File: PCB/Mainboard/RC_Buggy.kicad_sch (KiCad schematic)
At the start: 12 parts, among them SW1 SW_Push, SW2 SW_Push, U1 ESP32-S3-WROOM-1

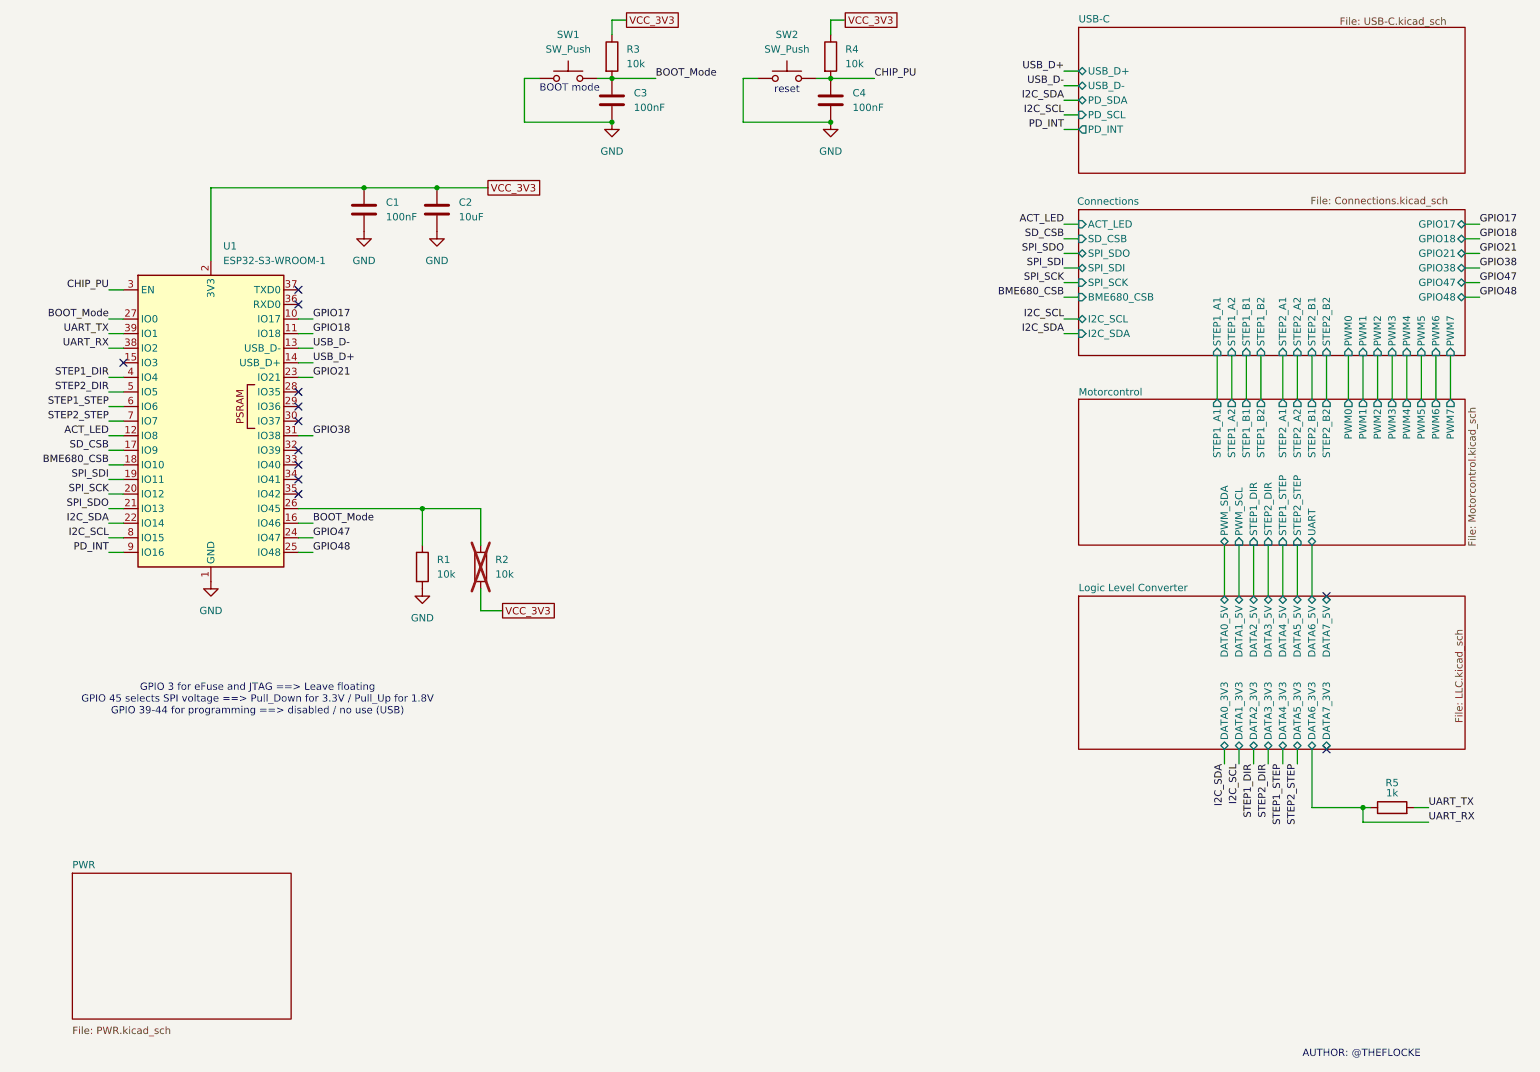
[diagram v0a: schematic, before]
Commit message: Fixed Grammar
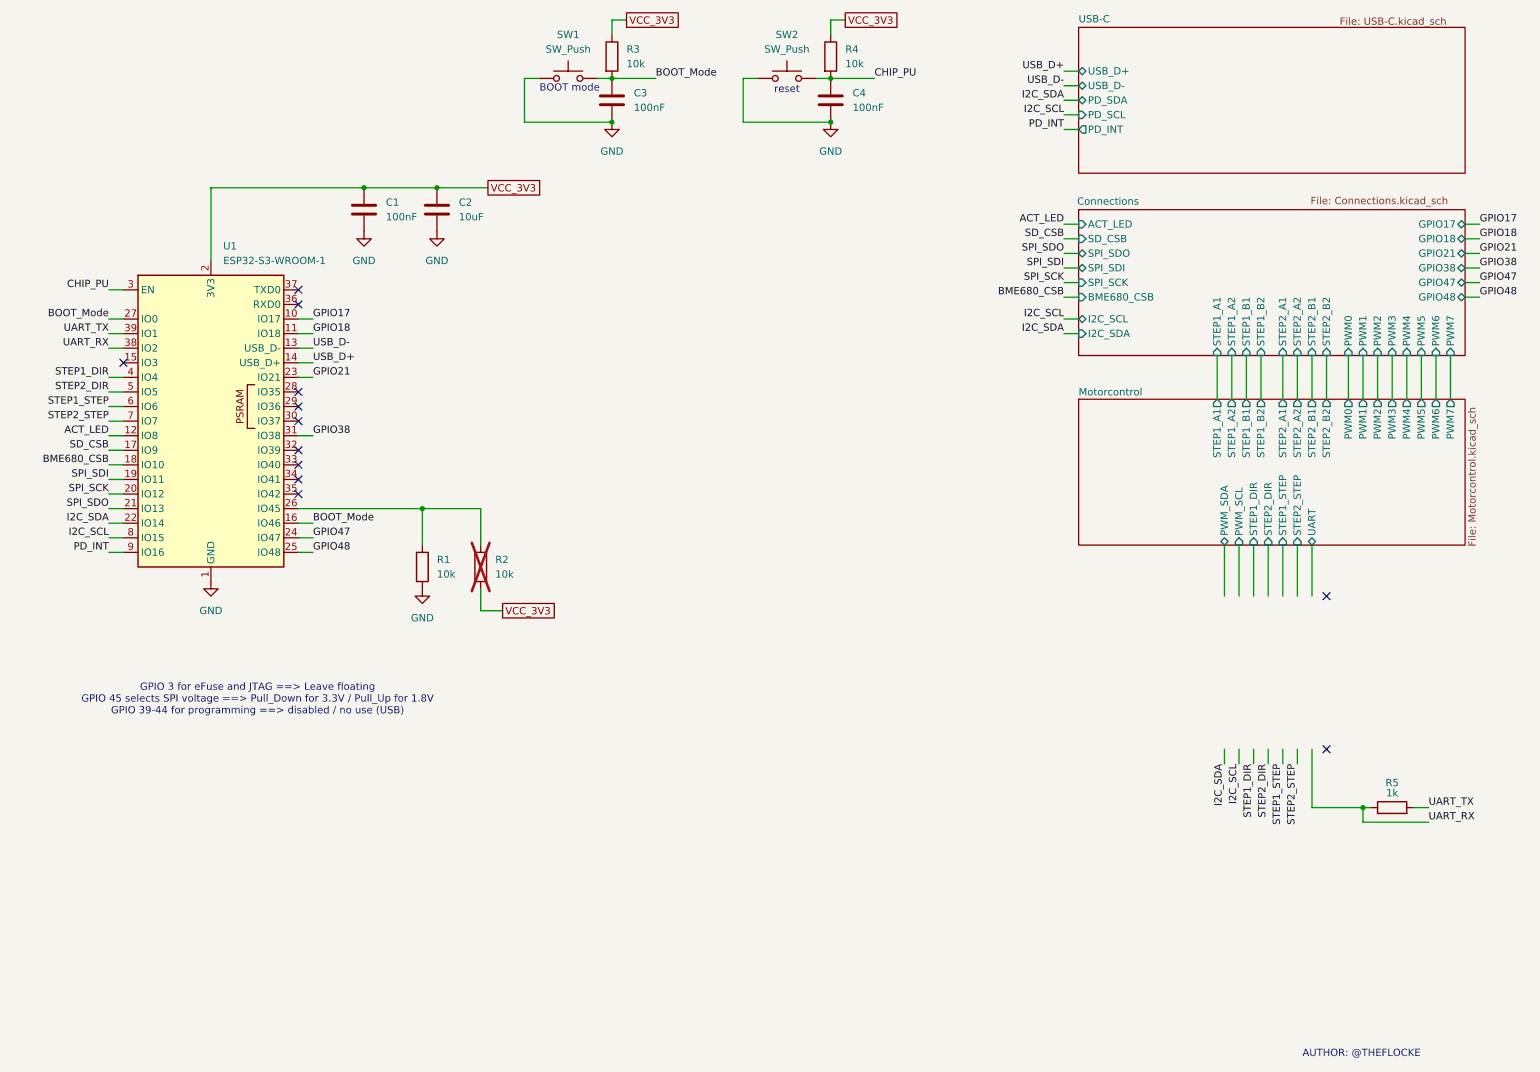
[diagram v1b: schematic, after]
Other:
- removed sheet Logic Level Converter
- removed sheet PWR
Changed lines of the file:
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@@
-	)
-	(sheet
-		(at 25.4 165.1)
-		(size 38.1 25.4)
-		(exclude_from_sim no)
-		(in_bom yes)
-		(on_board yes)
-		(dnp no)
-		(stroke
-			(width 0.1524)
-			(type solid)
-		)
-		(fill
-			(color 0 0 0 0.0000)
-		)
-		(property "Sheetname" "PWR"
-			(at 25.4 164.3884 0)
-			(effects
-				(font
-					(size 1.27 1.27)
-				)
-				(justify left bottom)
-			)
-		)
-		(property "Sheetfile" "PWR.kicad_sch"
-			(at 25.4 191.77 0)
-			(effects
-				(font
-					(size 1.27 1.27)
-				)
-				(justify left top)
-			)
-		)
-		(instances
-			(project "RC_Buggy"
-				(path "/95edd31c-9fee-4eef-843b-c880bdcf4bfe"
-					(page "3")
-				)
-			)
-		)
-	)
-	(sheet
-		(at 200.66 116.84)
-		(size 67.31 26.67)
-		(exclude_from_sim no)
-		(in_bom yes)
-		(on_board yes)
-		(dnp no)
-		(stroke
-			(width 0.1524)
-			(type solid)
-		)
-		(fill
-			(color 0 0 0 0.0000)
-		)
-		(property "Sheetname" "Logic Level Converter"
-			(at 200.66 116.1284 0)
-			(effects
-				(font
-					(size 1.27 1.27)
-				)
-				(justify left bottom)
-			)
-		)
-		(property "Sheetfile" "LLC.kicad_sch"
-			(at 266.192 138.938 90)
-			(effects
-				(font
-					(size 1.27 1.27)
-				)
-				(justify left top)
-			)
-		)
-		(pin "DATA2_5V" bidirectional
-			(at 231.14 116.84 90)
-			(effects
-				(font
-					(size 1.27 1.27)
-				)
-				(justify right)
-			)
-		)
-		(pin "DATA2_3V3" bidirectional
-			(at 231.14 143.51 270)
-			(effects
-				(font
-					(size 1.27 1.27)
-				)
-				(justify left)
-			)
-		)
-		(pin "DATA0_5V" bidirectional
-			(at 226.06 116.84 90)
-			(effects
-				(font
-					(size 1.27 1.27)
-				)
-				(justify right)
-			)
-		)
-		(pin "DATA0_3V3" bidirectional
-			(at 226.06 143.51 270)
-			(effects
-				(font
-					(size 1.27 1.27)
-				)
-				(justify left)
-			)
-		)
-		(pin "DATA7_3V3" bidirectional
-			(at 243.84 143.51 270)
-			(effects
-				(font
-					(size 1.27 1.27)
-				)
-				(justify left)
-			)
-		)
-		(pin "DATA6_3V3" bidirectional
-			(at 241.3 143.51 270)
-			(effects
-				(font
-					(size 1.27 1.27)
-				)
-				(justify left)
-			)
-		)
-		(pin "DATA1_3V3" bidirectional
-			(at 228.6 143.51 270)
-			(effects
-				(font
-					(size 1.27 1.27)
-				)
-				(justify left)
-			)
-		)
-		(pin "DATA3_3V3" bidirectional
-			(at 233.68 143.51 270)
-			(effects
-				(font
-					(size 1.27 1.27)
-				)
-				(justify left)
-			)
-		)
-		(pin "DATA5_3V3" bidirectional
-			(at 238.76 143.51 270)
-			(effects
-				(font
-					(size 1.27 1.27)
-				)
-				(justify left)
-			)
-		)
-		(pin "DATA4_3V3" bidirectional
-			(at 236.22 143.51 270)
-			(effects
-				(font
-					(size 1.27 1.27)
-				)
-				(justify left)
-			)
-		)
-		(pin "DATA4_5V" bidirectional
-			(at 236.22 116.84 90)
-			(effects
-				(font
-					(size 1.27 1.27)
-				)
-				(justify right)
-			)
-		)
-		(pin "DATA7_5V" bidirectional
-			(at 243.84 116.84 90)
-			(effects
-				(font
-					(size 1.27 1.27)
-				)
-				(justify right)
-			)
-		)
-		(pin "DATA6_5V" bidirectional
-			(at 241.3 116.84 90)
-			(effects
-				(font
-					(size 1.27 1.27)
-				)
-				(justify right)
-			)
-		)
-		(pin "DATA1_5V" bidirectional
-			(at 228.6 116.84 90)
-			(effects
-				(font
-					(size 1.27 1.27)
-				)
-				(justify right)
-			)
-		)
-		(pin "DATA3_5V" bidirectional
-			(at 233.68 116.84 90)
-			(effects
-				(font
-					(size 1.27 1.27)
-				)
-				(justify right)
-			)
-		)
-		(pin "DATA5_5V" bidirectional
-			(at 238.76 116.84 90)
-			(effects
-				(font
-					(size 1.27 1.27)
-				)
-				(justify right)
-			)
-		)
-		(instances
-			(project "RC_Buggy"
-				(path "/95edd31c-9fee-4eef-843b-c880bdcf4bfe"
-					(page "4")
-				)
-			)
-		)
 	)
 	(sheet

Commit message: upload images and deleted pcb new
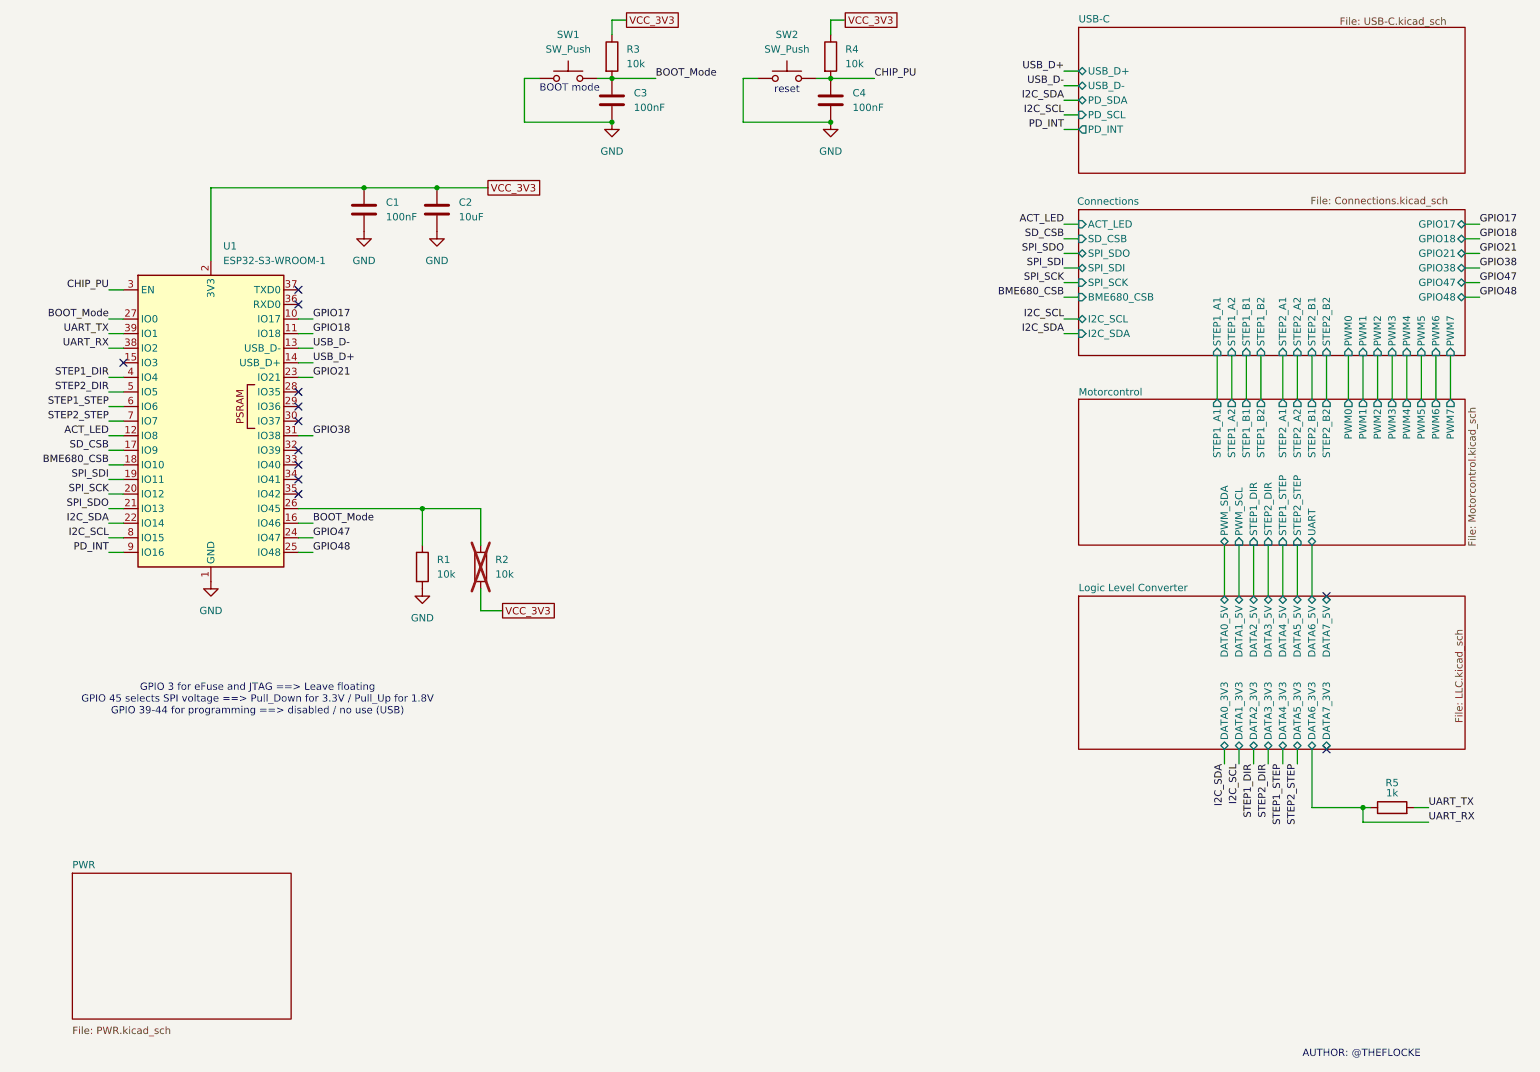
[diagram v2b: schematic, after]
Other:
- added sheet Logic Level Converter (LLC.kicad_sch)
- added sheet PWR (PWR.kicad_sch)
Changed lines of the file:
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@@
+	)
+	(sheet
+		(at 25.4 165.1)
+		(size 38.1 25.4)
+		(exclude_from_sim no)
+		(in_bom yes)
+		(on_board yes)
+		(dnp no)
+		(stroke
+			(width 0.1524)
+			(type solid)
+		)
+		(fill
+			(color 0 0 0 0.0000)
+		)
+		(property "Sheetname" "PWR"
+			(at 25.4 164.3884 0)
+			(effects
+				(font
+					(size 1.27 1.27)
+				)
+				(justify left bottom)
+			)
+		)
+		(property "Sheetfile" "PWR.kicad_sch"
+			(at 25.4 191.77 0)
+			(effects
+				(font
+					(size 1.27 1.27)
+				)
+				(justify left top)
+			)
+		)
+		(instances
+			(project "RC_Buggy"
+				(path "/95edd31c-9fee-4eef-843b-c880bdcf4bfe"
+					(page "3")
+				)
+			)
+		)
+	)
+	(sheet
+		(at 200.66 116.84)
+		(size 67.31 26.67)
+		(exclude_from_sim no)
+		(in_bom yes)
+		(on_board yes)
+		(dnp no)
+		(stroke
+			(width 0.1524)
+			(type solid)
+		)
+		(fill
+			(color 0 0 0 0.0000)
+		)
+		(property "Sheetname" "Logic Level Converter"
+			(at 200.66 116.1284 0)
+			(effects
+				(font
+					(size 1.27 1.27)
+				)
+				(justify left bottom)
+			)
+		)
+		(property "Sheetfile" "LLC.kicad_sch"
+			(at 266.192 138.938 90)
+			(effects
+				(font
+					(size 1.27 1.27)
+				)
+				(justify left top)
+			)
+		)
+		(pin "DATA2_5V" bidirectional
+			(at 231.14 116.84 90)
+			(effects
+				(font
+					(size 1.27 1.27)
+				)
+				(justify right)
+			)
+		)
+		(pin "DATA2_3V3" bidirectional
+			(at 231.14 143.51 270)
+			(effects
+				(font
+					(size 1.27 1.27)
+				)
+				(justify left)
+			)
+		)
+		(pin "DATA0_5V" bidirectional
+			(at 226.06 116.84 90)
+			(effects
+				(font
+					(size 1.27 1.27)
+				)
+				(justify right)
+			)
+		)
+		(pin "DATA0_3V3" bidirectional
+			(at 226.06 143.51 270)
+			(effects
+				(font
+					(size 1.27 1.27)
+				)
+				(justify left)
+			)
+		)
+		(pin "DATA7_3V3" bidirectional
+			(at 243.84 143.51 270)
+			(effects
+				(font
+					(size 1.27 1.27)
+				)
+				(justify left)
+			)
+		)
+		(pin "DATA6_3V3" bidirectional
+			(at 241.3 143.51 270)
+			(effects
+				(font
+					(size 1.27 1.27)
+				)
+				(justify left)
+			)
+		)
+		(pin "DATA1_3V3" bidirectional
+			(at 228.6 143.51 270)
+			(effects
+				(font
+					(size 1.27 1.27)
+				)
+				(justify left)
+			)
+		)
+		(pin "DATA3_3V3" bidirectional
+			(at 233.68 143.51 270)
+			(effects
+				(font
+					(size 1.27 1.27)
+				)
+				(justify left)
+			)
+		)
+		(pin "DATA5_3V3" bidirectional
+			(at 238.76 143.51 270)
+			(effects
+				(font
+					(size 1.27 1.27)
+				)
+				(justify left)
+			)
+		)
+		(pin "DATA4_3V3" bidirectional
+			(at 236.22 143.51 270)
+			(effects
+				(font
+					(size 1.27 1.27)
+				)
+				(justify left)
+			)
+		)
+		(pin "DATA4_5V" bidirectional
+			(at 236.22 116.84 90)
+			(effects
+				(font
+					(size 1.27 1.27)
+				)
+				(justify right)
+			)
+		)
+		(pin "DATA7_5V" bidirectional
+			(at 243.84 116.84 90)
+			(effects
+				(font
+					(size 1.27 1.27)
+				)
+				(justify right)
+			)
+		)
+		(pin "DATA6_5V" bidirectional
+			(at 241.3 116.84 90)
+			(effects
+				(font
+					(size 1.27 1.27)
+				)
+				(justify right)
+			)
+		)
+		(pin "DATA1_5V" bidirectional
+			(at 228.6 116.84 90)
+			(effects
+				(font
+					(size 1.27 1.27)
+				)
+				(justify right)
+			)
+		)
+		(pin "DATA3_5V" bidirectional
+			(at 233.68 116.84 90)
+			(effects
+				(font
+					(size 1.27 1.27)
+				)
+				(justify right)
+			)
+		)
+		(pin "DATA5_5V" bidirectional
+			(at 238.76 116.84 90)
+			(effects
+				(font
+					(size 1.27 1.27)
+				)
+				(justify right)
+			)
+		)
+		(instances
+			(project "RC_Buggy"
+				(path "/95edd31c-9fee-4eef-843b-c880bdcf4bfe"
+					(page "4")
+				)
+			)
+		)
 	)
 	(sheet
